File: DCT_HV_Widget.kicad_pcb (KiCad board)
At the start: 2 copper layers, 53.9 x 74.6 mm, 27 parts, among them J1 Control Voltage, J2 Bench Power Supply, J3 High Voltage, Q1 ZXTN10150D, U1 LT1468CS8-PBF, U2 OC150G

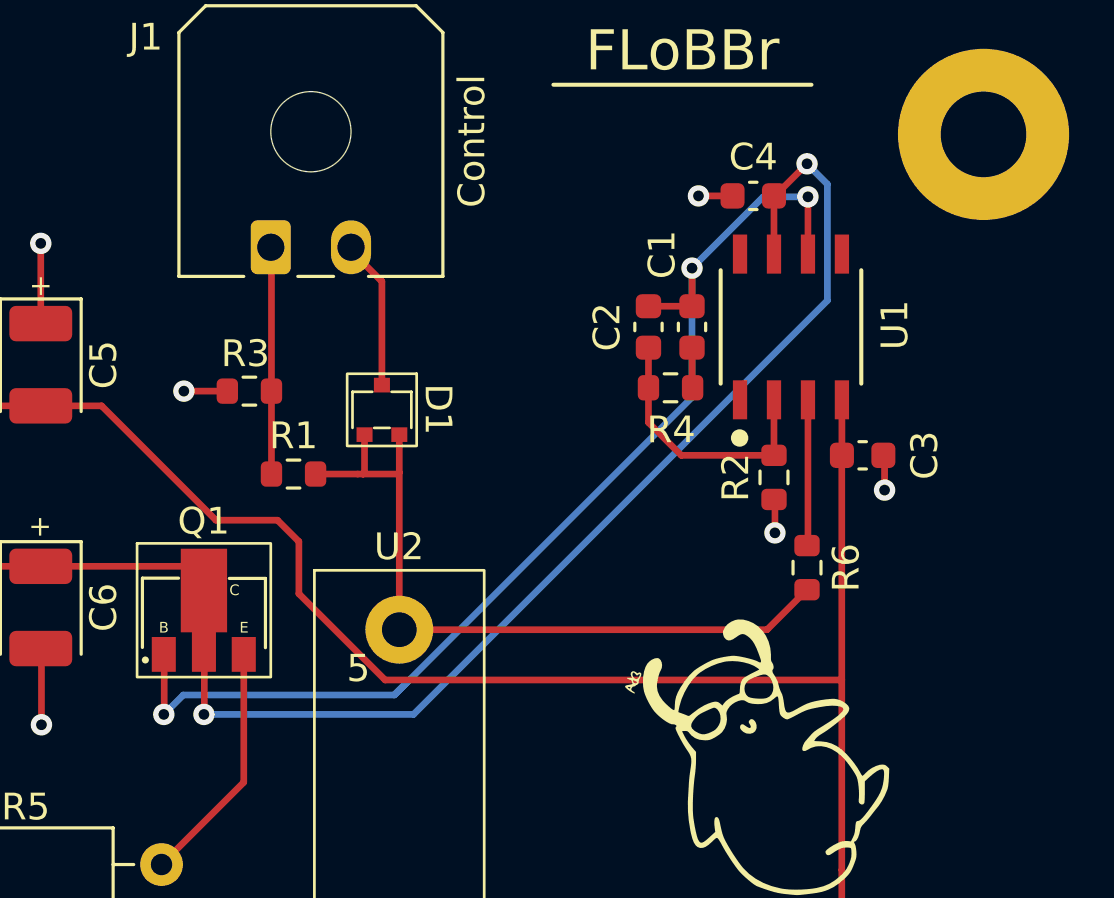
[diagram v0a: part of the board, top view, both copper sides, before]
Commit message: Ready for fab. FLoBBr rev1
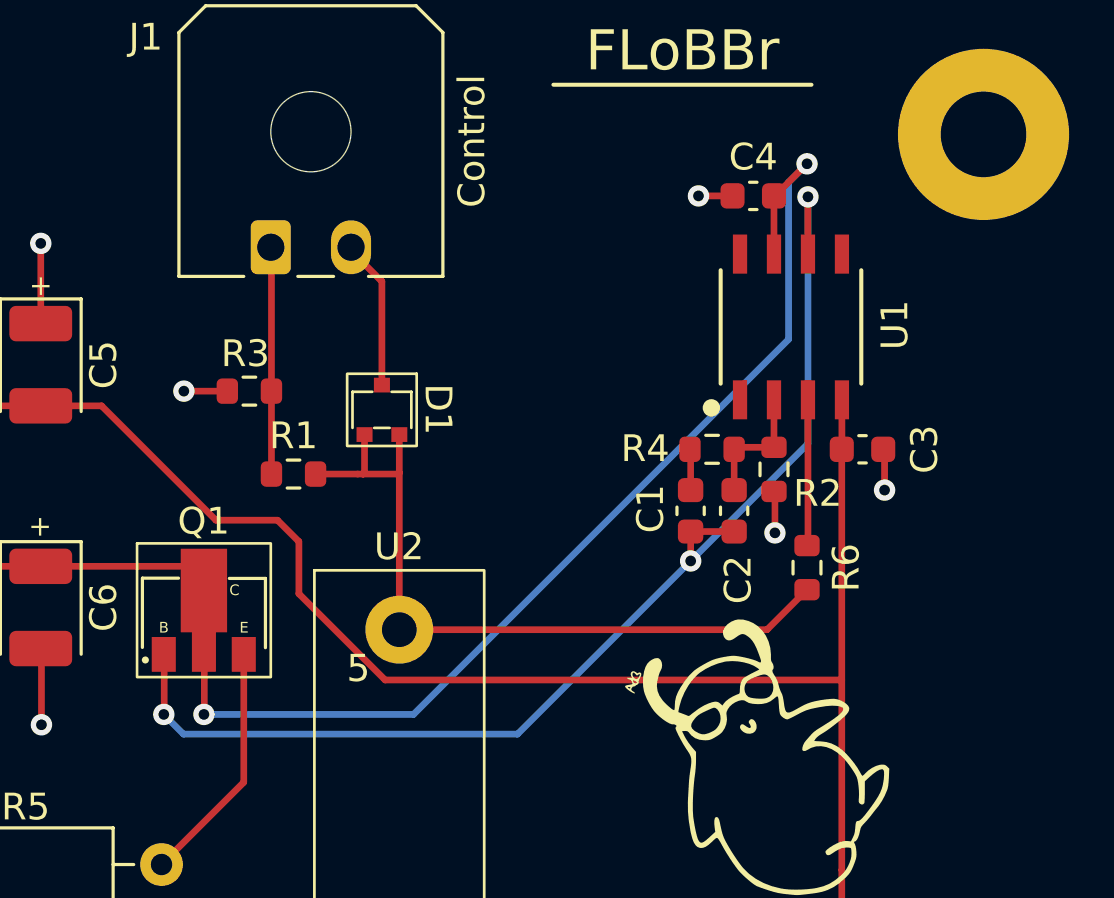
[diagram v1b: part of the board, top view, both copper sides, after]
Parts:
- moved C2 7.58 mm to (172.9, 88.6), turned to -90 degrees
- moved C1 6.88 mm to (171.2, 88.6), turned to -90 degrees
- moved R4 2.78 mm to (172.1, 86.3), turned to 180 degrees
- moved R2 0.30 mm to (174.4, 87.0)
- moved C3 0.23 mm to (177.7, 86.3)
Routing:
- net Net-(C2-Pad1): track 9.91 -> 4.82 mm
- net Net-(C1-Pad2): track 43.0 -> 45.2 mm
- net /VP6: track 52.2 -> 51.6 mm
